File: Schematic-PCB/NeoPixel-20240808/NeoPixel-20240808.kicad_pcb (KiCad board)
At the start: 2 copper layers, 102 x 102 mm, 37 parts, among them J1 Conn_01x05_Pin

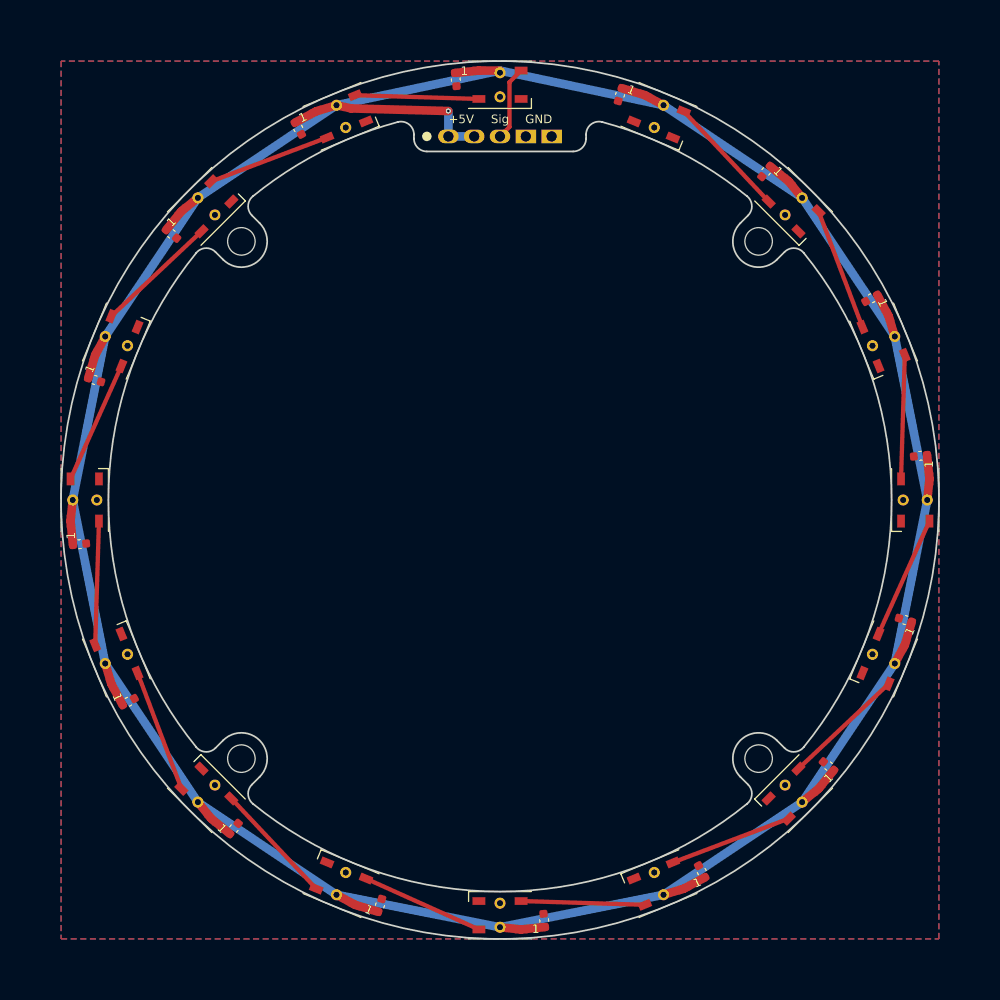
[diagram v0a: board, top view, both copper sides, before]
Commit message: update: NeoPixel基板の回路とPCBを完成させた
回路は大丈夫だと思う、PCBをしっかりDRお願い
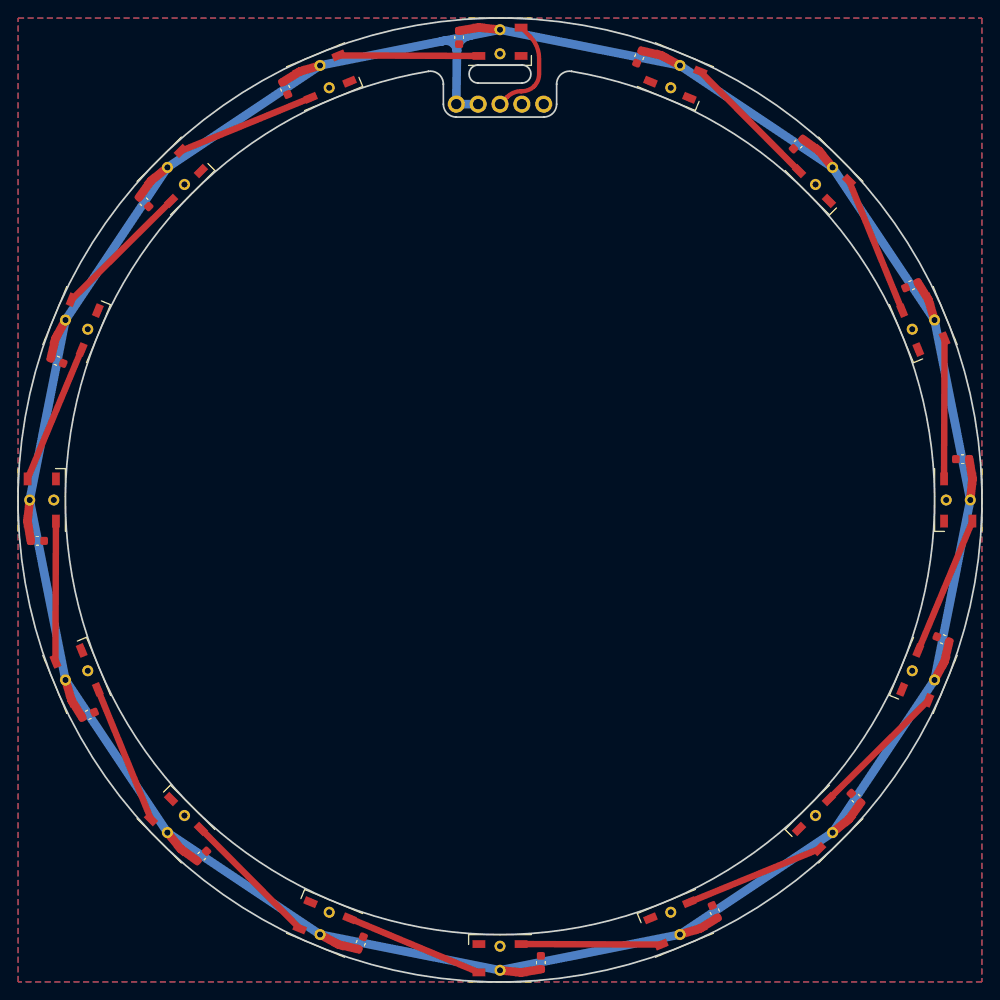
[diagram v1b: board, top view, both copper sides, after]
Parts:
- removed REF** (x4): MountingHole_3.2mm_M3, MountingHole:MountingHole_3.2mm_M3
- moved D10 5.00 mm to (20.4, 49.2)
- moved D12 5.00 mm to (49.2, 20.4)
- moved D14 5.00 mm to (49.2, -20.4)
- moved D16 5.00 mm to (20.4, -49.2)
- moved D2 5.00 mm to (-20.4, -49.2)
- moved D4 5.00 mm to (-49.2, -20.4)
- moved D6 5.00 mm to (-49.2, 20.4)
- moved D8 5.00 mm to (-20.4, 49.2)
- moved D11 5.00 mm to (37.7, 37.7)
- moved D15 5.00 mm to (37.7, -37.7)
- moved D3 5.00 mm to (-37.7, -37.7)
- moved D7 5.00 mm to (-37.7, 37.7)
- moved D1 5.00 mm to (0.00, -53.2)
- moved D13 5.00 mm to (53.2, 0.00)
- moved D5 5.00 mm to (-53.2, 0.00)
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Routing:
- net +5V: track 412.9 -> 431.4 mm, vias 1 -> 0
- net NeoPixel_PWM: track 8.66 -> 12.3 mm
- net Net-(D7-DOUT): track 14.4 -> 16.3 mm
- net Net-(D3-DOUT): track 14.4 -> 16.3 mm
- net Net-(D15-DOUT): track 14.4 -> 16.3 mm
- net Net-(D11-DOUT): track 14.4 -> 16.3 mm
- net Net-(D6-DOUT): track 14.4 -> 16.3 mm
- net Net-(D2-DOUT): track 14.4 -> 16.3 mm
- net Net-(D14-DOUT): track 14.4 -> 16.3 mm
- net Net-(D10-DOUT): track 14.4 -> 16.3 mm
- net Net-(D5-DOUT): track 14.4 -> 16.3 mm
- net Net-(D13-DOUT): track 14.4 -> 16.3 mm
- net Net-(D10-DIN): track 14.4 -> 16.3 mm
- net Net-(D1-DOUT): track 14.4 -> 16.3 mm
- net Net-(D8-DOUT): track 14.4 -> 16.3 mm
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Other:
- board size 102 x 102 mm -> 112 x 112 mm
- board text removed: "+5V"
- board text removed: "GND"
- board text removed: "Sig"
